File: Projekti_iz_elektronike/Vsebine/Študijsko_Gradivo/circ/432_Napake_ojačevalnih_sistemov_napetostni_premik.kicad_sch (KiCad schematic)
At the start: 8 parts, among them U1 LM358

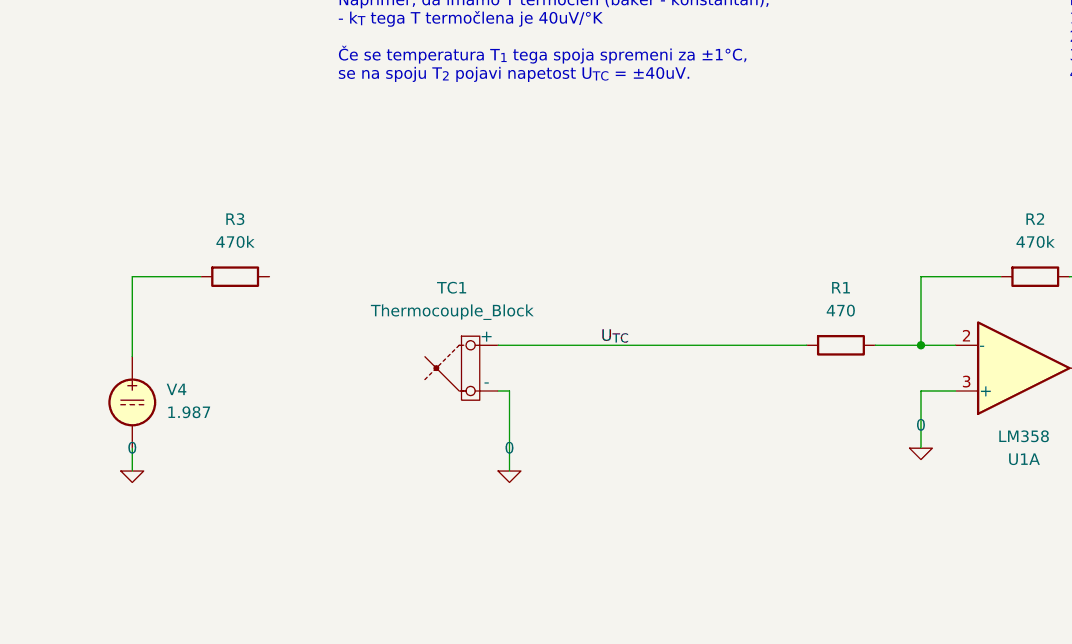
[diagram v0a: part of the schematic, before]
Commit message: thom
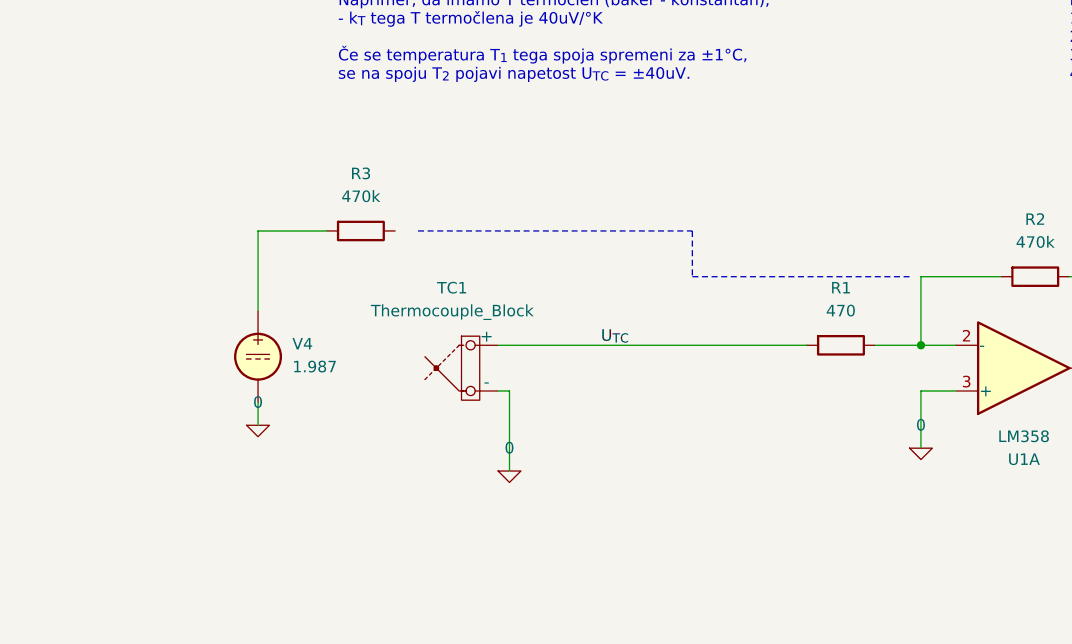
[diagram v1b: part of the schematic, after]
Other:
- moved on the sheet: R3, V4

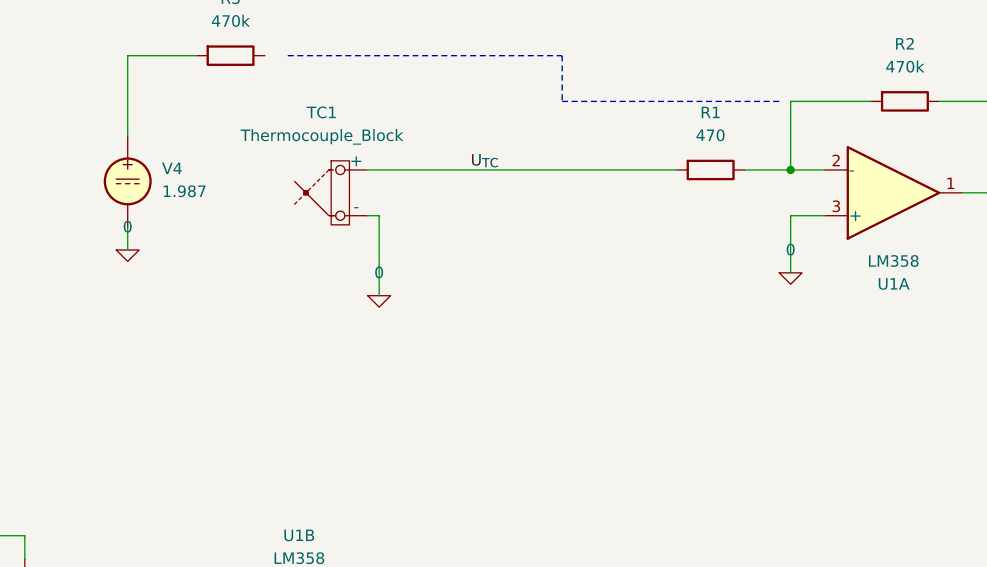
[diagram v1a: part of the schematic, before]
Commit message: GPT_agent
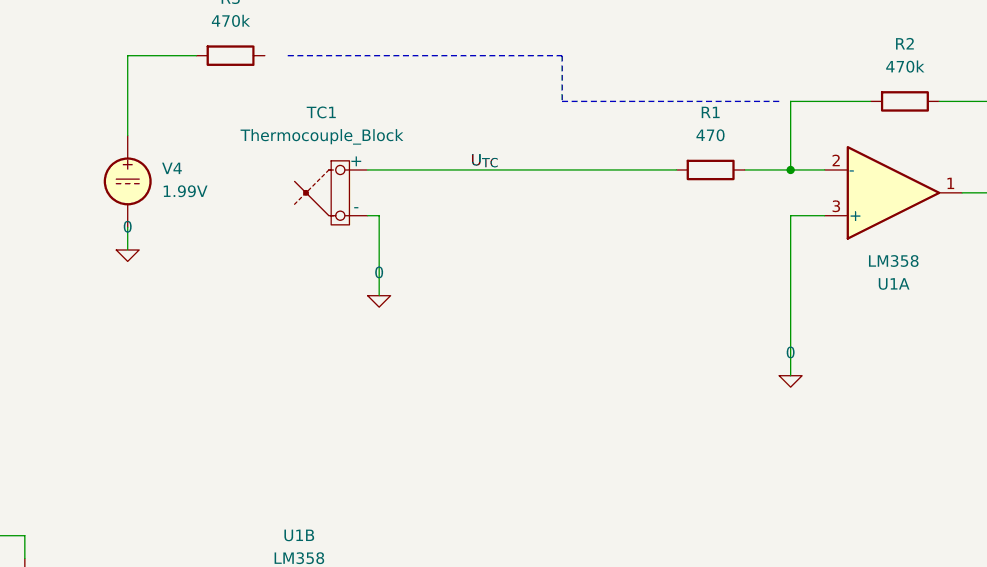
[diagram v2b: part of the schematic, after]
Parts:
- V4: value 1.987 -> 1.99V
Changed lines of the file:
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@@
+	(wire
+		(pts
+			(xy 123.19 68.58) (xy 127 68.58)
+		)
+		(stroke
+			(width 0)
+			(type default)
+		)
+	)
 	(wire
 		(pts
@@
 	(wire
 		(pts
-			(xy 123.19 68.58) (xy 123.19 74.93)
-		)
-		(stroke
-			(width 0)
-			(type default)
-		)
-	)
-	(wire
-		(pts
 			(xy 57.15 50.8) (xy 49.53 50.8)
 		)
@@
 		)
 	)
+	(wire
+		(pts
+			(xy 123.19 68.58) (xy 123.19 86.36)
+		)
+		(stroke
+			(width 0)
+			(type default)
+		)
+	)
 	(polyline
 		(pts
@@
 		(pts
 			(xy 146.05 55.88) (xy 146.05 66.04)
-		)
-		(stroke
-			(width 0)
-			(type default)
-		)
-	)
-	(wire
-		(pts
-			(xy 127 68.58) (xy 123.19 68.58)
 		)
 		(stroke
@@
 			)
 		)
-		(property "Value" "1.987"
+		(property "Value" "1.99V"
 			(at 53.34 65.9102 0)
 			(effects
@@
 	(symbol
 		(lib_id "Simulation_SPICE:0")
-		(at 123.19 74.93 0)
+		(at 123.19 86.36 0)
 		(unit 1)
 		(exclude_from_sim no)
@@
 		(fields_autoplaced yes)
 		(property "Reference" "#GND01"
-			(at 123.19 77.47 0)
+			(at 123.19 88.9 0)
 			(effects
 				(font
@@
 		)
 		(property "Value" "0"
-			(at 123.19 72.39 0)
+			(at 123.19 83.82 0)
 			(effects
 				(font
@@
 		)
 		(property "Footprint" ""
-			(at 123.19 74.93 0)
+			(at 123.19 86.36 0)
 			(effects
 				(font
@@
 		)
 		(property "Datasheet" "~"
-			(at 123.19 74.93 0)
+			(at 123.19 86.36 0)
 			(effects
 				(font
@@
 		)
 		(property "Description" ""
-			(at 123.19 74.93 0)
-			(effects
-				(font
+			(at 123.19 86.36 0)
+			(effects
+				(font
